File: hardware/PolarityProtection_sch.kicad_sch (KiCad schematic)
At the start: 18 parts, among them IC1 LM74502HDDFR, Q1 NVMFWS1D7N04XMT1G, Q4 NVMFWS1D7N04XMT1G

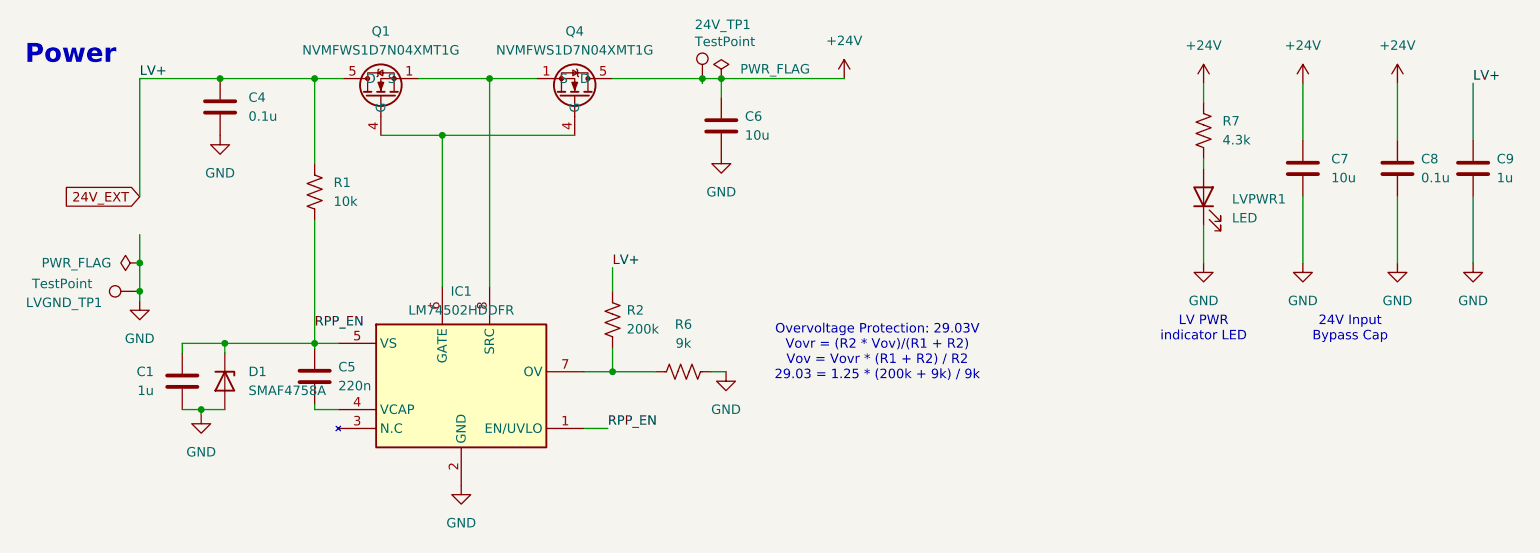
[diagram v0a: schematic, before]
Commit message: Rev B schematic Review with new IC
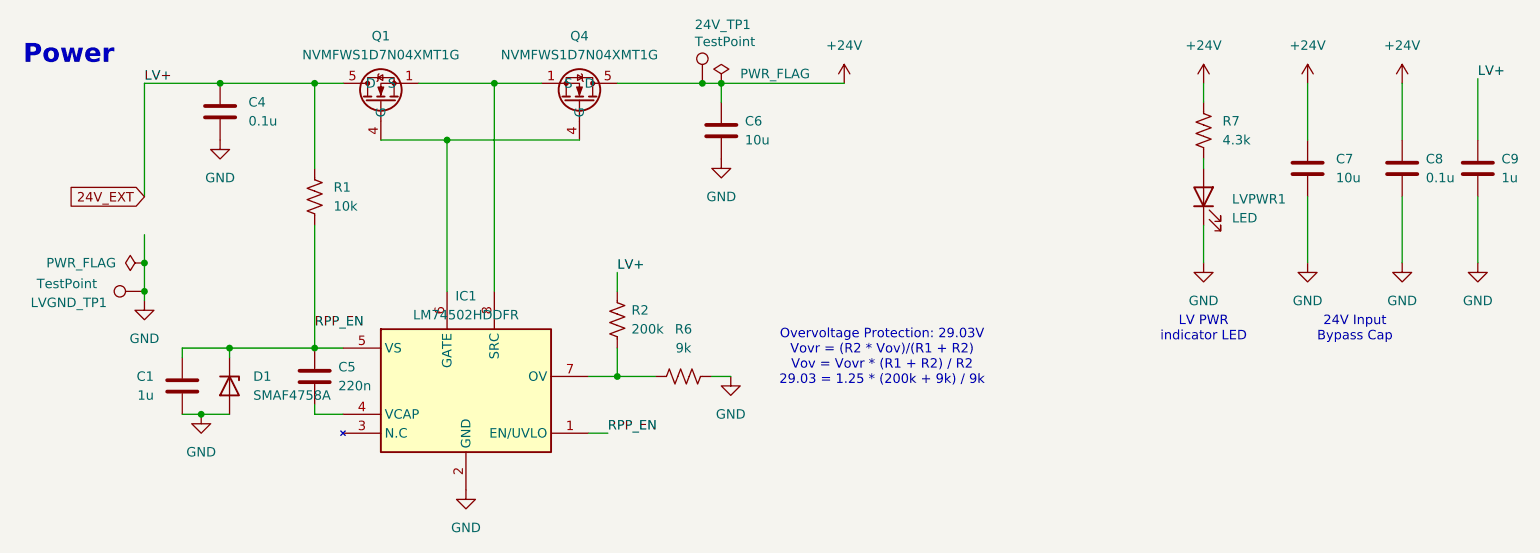
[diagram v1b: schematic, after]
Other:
- moved on the sheet: C1, C4, C6, C7, C8, C9, D1, IC1, LVGND_TP1, Q1, Q4, R1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
